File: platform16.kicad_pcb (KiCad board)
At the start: 2 copper layers, 111.7 x 86.2 mm, 112 parts, among them CN1 PJ-342, CN2 PJ-342, CN3 PJ-342, IC1 PAM8908JER, J2 Conn_01x03, J4 SM03B-SRSS-TB, Q1 SS8050, Q3 SS8050, SW2 TS-1095PS-A165B2-C3D2, SW3 TS-1095PS-A165B2-C3D2, U1 RP2350_60QFN, U2 NCP1117-3.3_SOT223, U3 W25Q128JVS, U4 CD74HC4067SM, U5 PCM5100A, Y1 ABM8-272-T3

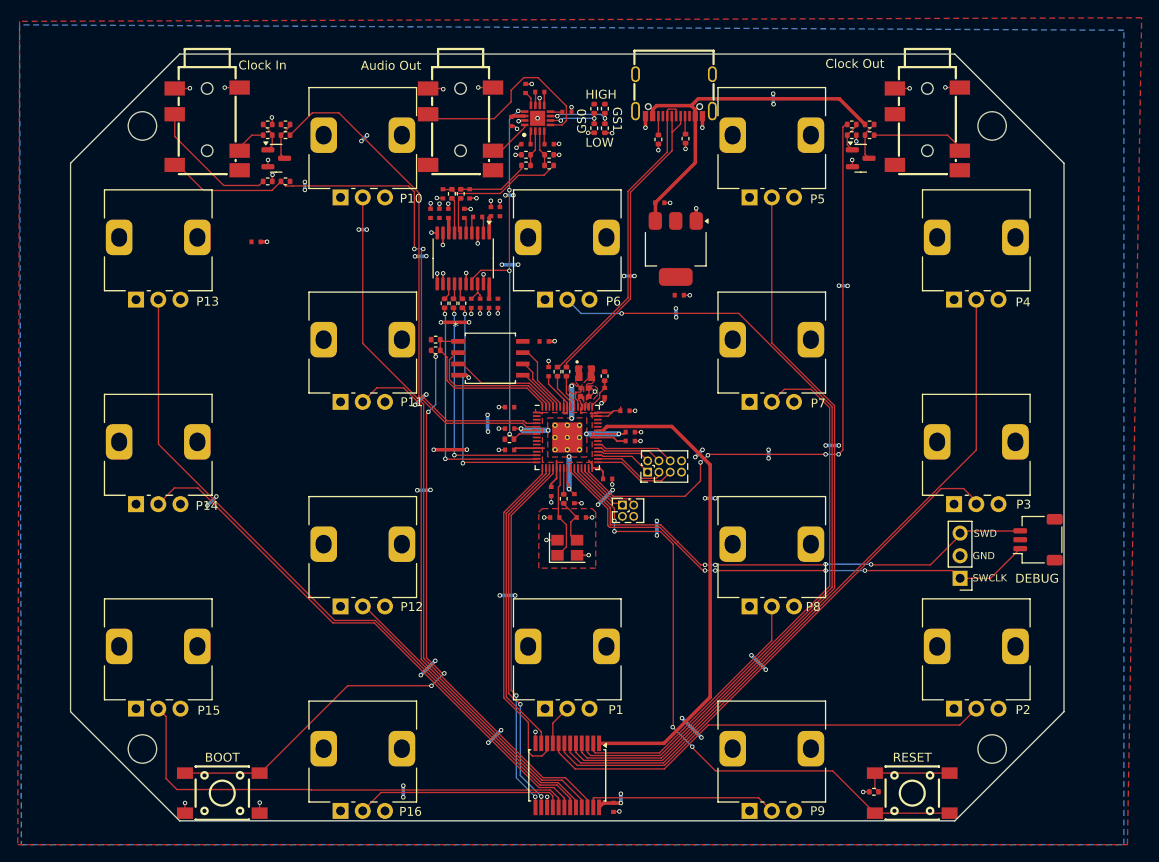
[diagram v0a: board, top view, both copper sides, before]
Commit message: tweaks
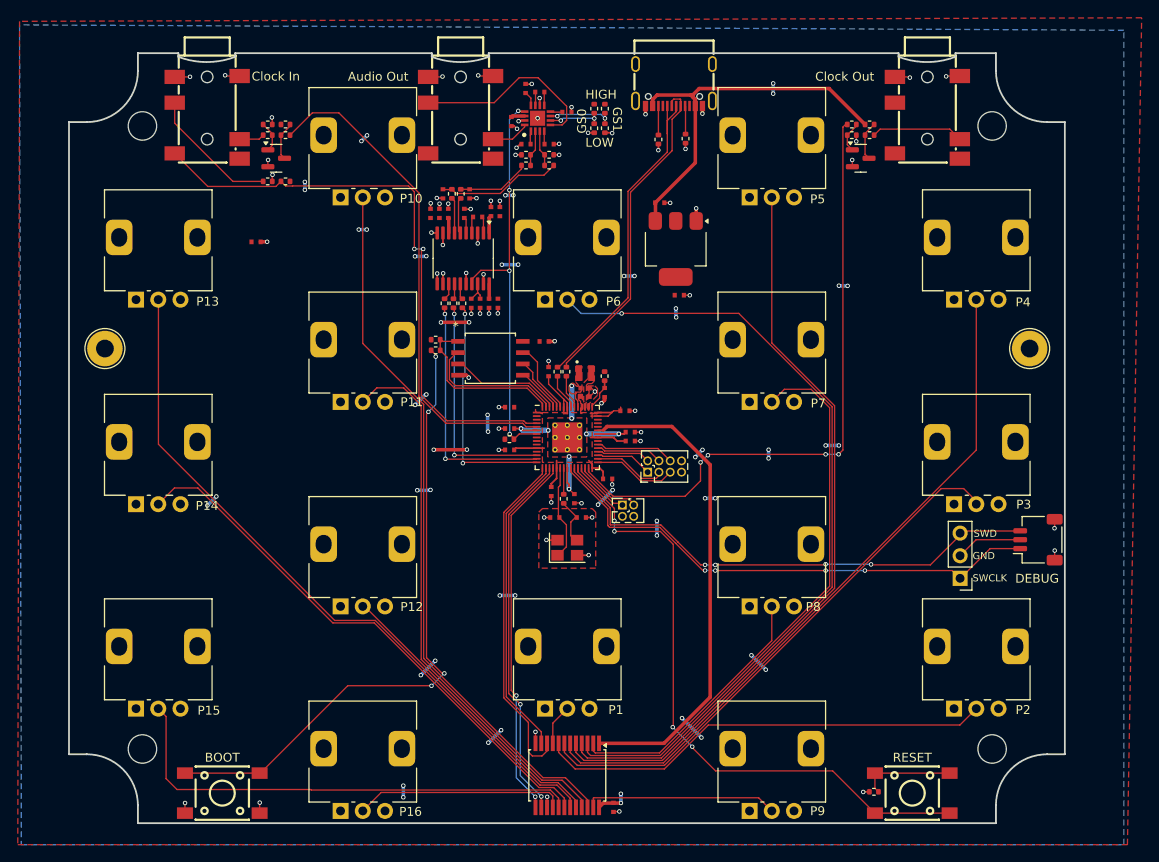
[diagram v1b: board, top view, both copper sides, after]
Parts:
- added TP1: TestPoint, TestPoint:TestPoint_THTPad_D4.0mm_Drill2.0mm, F.Cu at (96.5, 95.0)
- added TP2: TestPoint, TestPoint:TestPoint_THTPad_D4.0mm_Drill2.0mm, F.Cu at (200.5, 95.0)
- moved CN1 1.30 mm to (108.0, 69.0)
- moved CN2 1.30 mm to (189.0, 69.0)
- moved CN3 1.30 mm to (136.5, 69.0)
- moved USB1 1.14 mm to (160.5, 65.4)
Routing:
- net GND: track 73.6 -> 83.0 mm, vias 78 -> 80
- net VBUS: track 41.0 -> 44.2 mm
- net /USB_D-: track 34.7 -> 37.1 mm
- net /USB_D+: track 36.2 -> 38.1 mm
- net /HEADPHONE_R: track 23.2 -> 21.7 mm
- net /CC2: track 1.86 -> 3.26 mm
- net /CC1: track 1.82 -> 3.18 mm
- net /CLOCK_IN_HV: track 4.09 -> 2.84 mm
- net /HEADPHONE_L: track 5.13 -> 4.35 mm
- net /CLOCK_OUT_HV: track 11.1 -> 10.4 mm
- net /CLOCK_RING_PULLDOWN: track 14.4 -> 15.0 mm
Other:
- board size 111.7 x 86.2 mm -> 112 x 86.6 mm
- board text added: "DEBUG"
- board text added: "TODO: * Add test points, especially for alligator clips"
- board text removed: "TODO: lower the amplification for headphones & line out?"

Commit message: another iteration
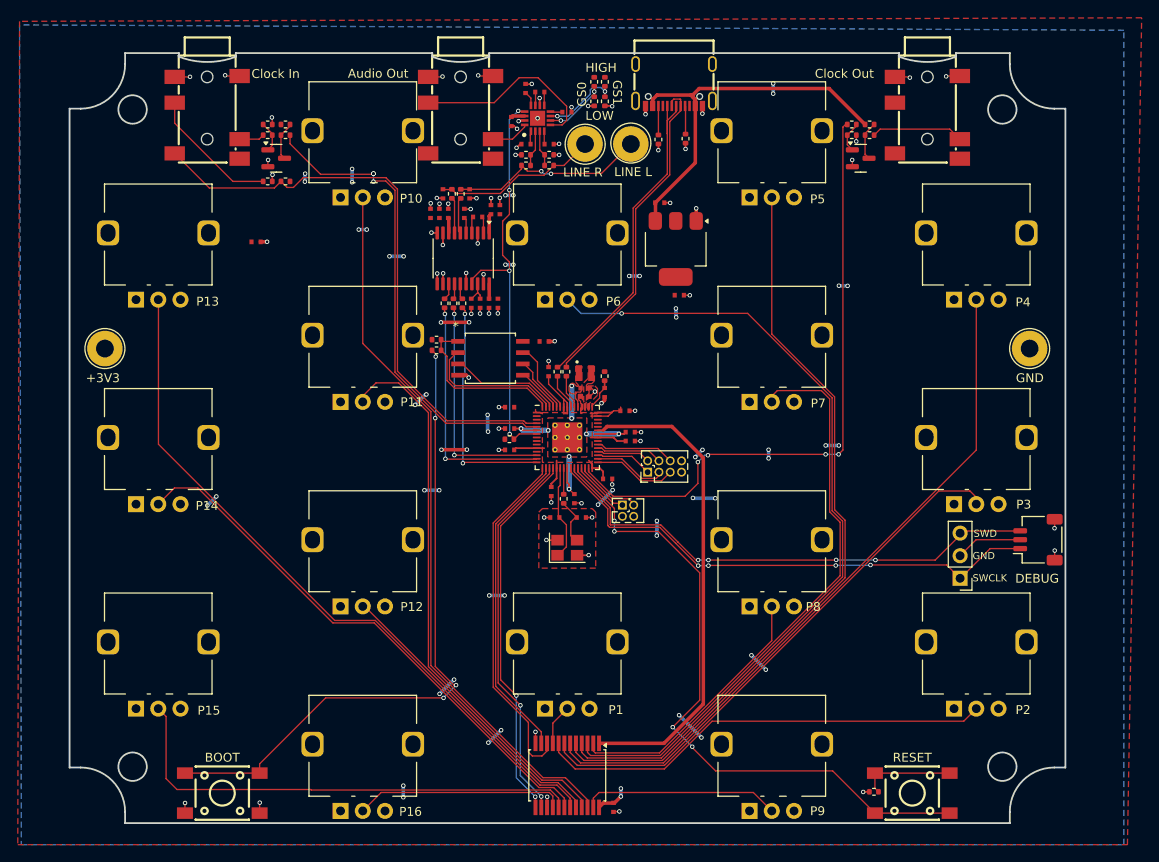
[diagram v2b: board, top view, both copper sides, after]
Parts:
- removed REF** (x4): MountingHole_3.2mm_M3, MountingHole:MountingHole_3.2mm_M3
- added TP3: TestPoint, TestPoint:TestPoint_THTPad_D4.0mm_Drill2.0mm, F.Cu at (155.7, 71.9)
- added TP4: TestPoint, TestPoint:TestPoint_THTPad_D4.0mm_Drill2.0mm, F.Cu at (150.5, 72.0)
- moved R14 3.02 mm to (151.5, 65.0)
- moved R15 3.02 mm to (152.7, 65.0)
- moved R16 3.02 mm to (151.5, 67.2)
- moved R17 3.02 mm to (152.7, 67.2)
- moved C33 0.22 mm to (139.9, 79.4)
- moved C37 0.22 mm to (140.9, 79.4)
- moved R1 0.10 mm to (133.8, 94.0)
- moved R6 0.10 mm to (133.8, 95.2)
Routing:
- net /LINE_L: track 8.17 -> 22.5 mm, vias 0 -> 2
- net /LINE_R: track 14.0 -> 18.5 mm
- net /~{USB_BOOT}: track 71.8 -> 74.2 mm
- net +3V3: track 78.6 -> 81.0 mm
- net /RUN: track 71.8 -> 74.2 mm
- net /CLOCK_IN_3V3: track 56.8 -> 54.6 mm, vias 0 -> 3
- net /P5: track 85.4 -> 87.0 mm
- net /P6: track 92.5 -> 94.0 mm
- net /GAIN_SELECT1: track 7.59 -> 9.12 mm
- net /GAIN_SELECT0: track 6.23 -> 7.60 mm
- net /P7: track 64.3 -> 65.5 mm
- net /S3: track 41.2 -> 42.2 mm
- net /S1: track 34.4 -> 35.4 mm
- net /S0: track 38.3 -> 39.2 mm
- net /S2: track 41.7 -> 42.6 mm
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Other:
- outline, holes or cut-outs redrawn
- board text added: "+3V3"
- board text added: "LINE L"
- board text added: "LINE R"
- board text added: "TODO: * Add rounded edges & mouse bytes to pick between no/3d printed case vs 1590BB?"
- board text removed: "TODO: * Add test points, especially for alligator clips"
